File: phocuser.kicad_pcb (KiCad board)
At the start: 2 copper layers, 35 x 40 mm, 52 parts, among them J1 Conn_01x04_Male, J2 Conn_ARM_JTAG_SWD_10, J3 Conn_01x02_Male, J4 DX07S016JA1R1500, J5 Accessory 0, J6 Accessory 1, J7 Accessory 2, U1 HolyIot-18010, U2 TMC2130-LA, U3 FT231XQ

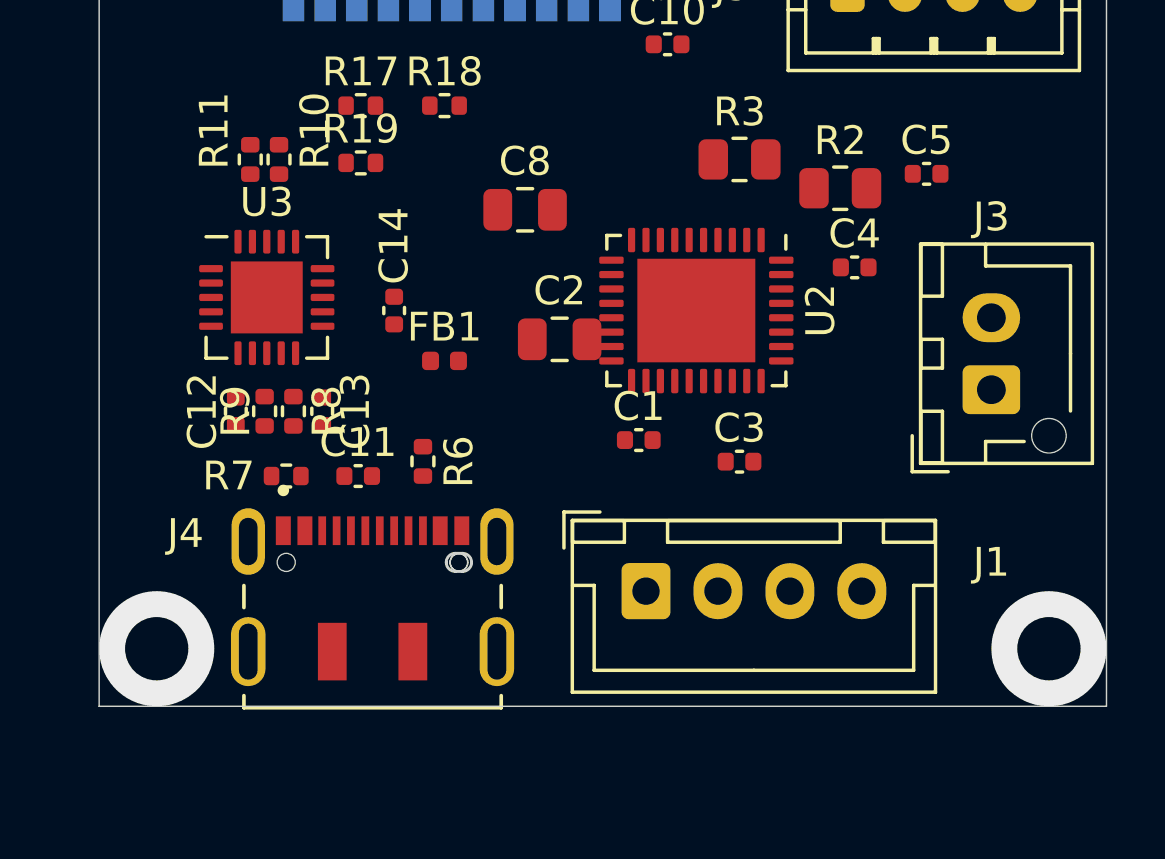
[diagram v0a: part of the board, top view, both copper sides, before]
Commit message: checkin
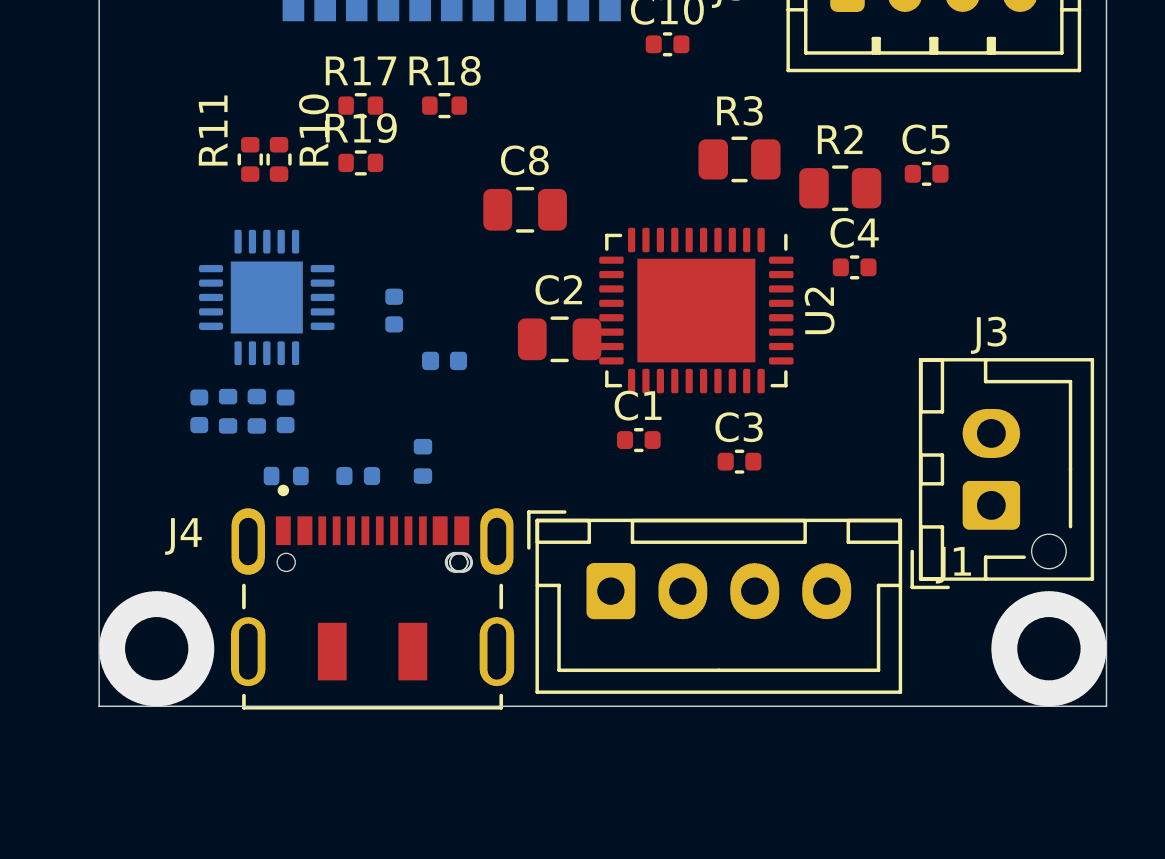
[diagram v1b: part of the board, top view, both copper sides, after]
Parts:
- C11, C12, C13, C14, FB1, R6, R7, R8, R9, U3: moved to B.Cu
- moved J3 4.02 mm to (196.0, 98.0)
- moved C12 1.27 mm to (168.5, 94.8), turned to 270 degrees
- moved C13 1.27 mm to (171.5, 94.8), turned to 90 degrees
- moved R8 1.27 mm to (170.5, 94.8), turned to 90 degrees
- moved R9 1.27 mm to (169.5, 94.8), turned to 90 degrees
- moved J1 1.22 mm to (182.8, 101.0)
- turned C14 to 90 degrees
- turned R6 to 270 degrees

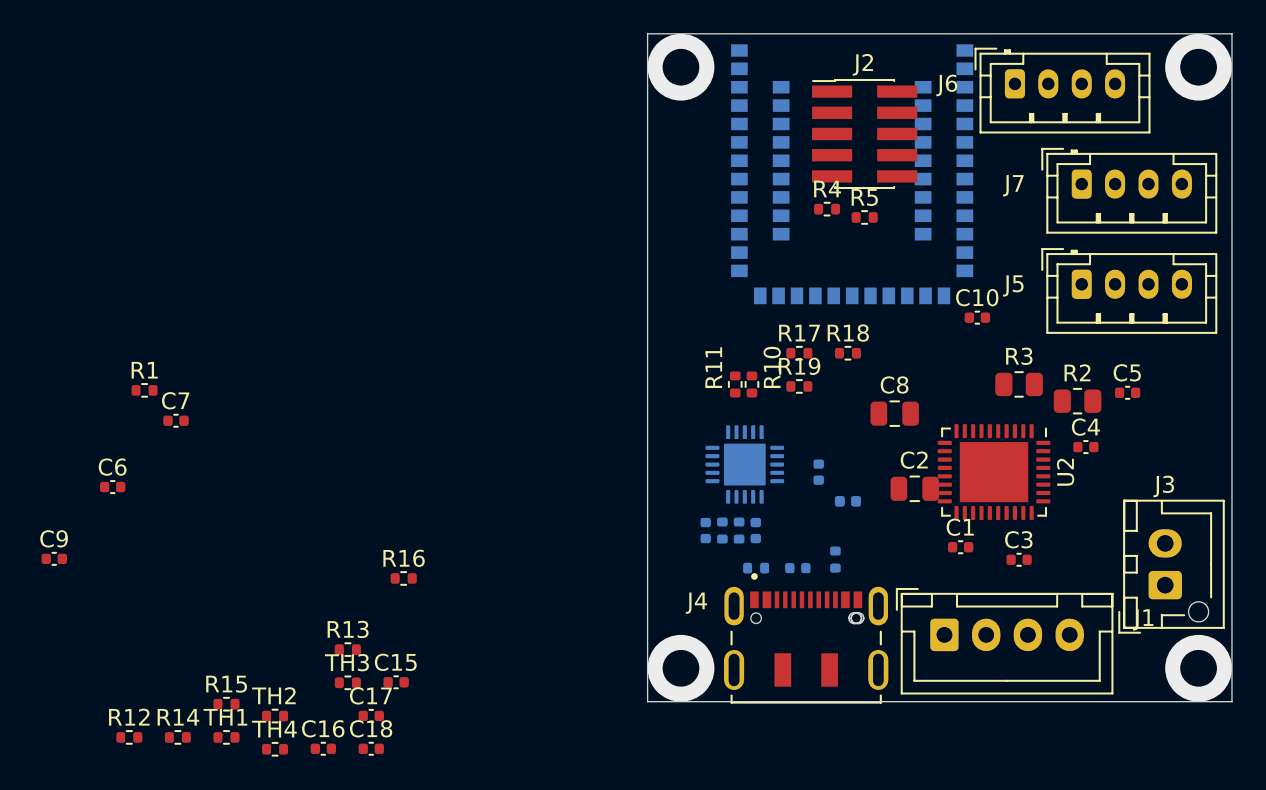
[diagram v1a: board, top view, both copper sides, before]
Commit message: Layout incremental checkin
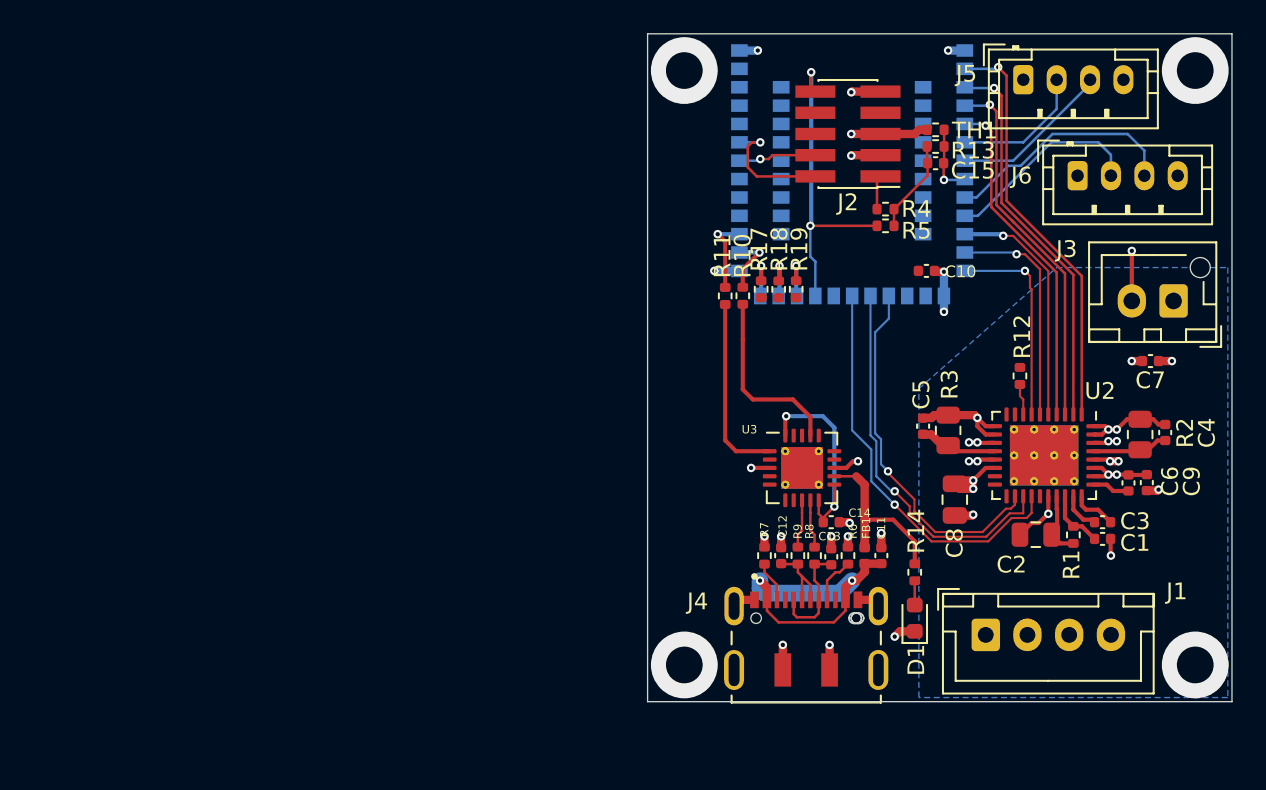
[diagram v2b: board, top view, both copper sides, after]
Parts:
- removed C16, C17, C18: 100nf, Capacitor_SMD:C_0402_1005Metric
- removed J7: Accessory 2, Connector_JST:JST_PH_B4B-PH-K_1x04_P2.00mm_Vertical
- removed R15, R16: 47k, Resistor_SMD:R_0402_1005Metric
- removed TH2, TH3, TH4: Thermistor_NTC, Resistor_SMD:R_0402_1005Metric
- added D1: LED, LED_SMD:LED_0603_1608Metric, F.Cu at (181.0, 100.0)
- C11, C12, C13, C14, FB1, R6, R7, R8, R9: moved to F.Cu
- R14: value 47k -> 470
- U2: footprint Package_DFN_QFN:QFN-36-1EP_5x6mm_P0.5mm_EP3.6x4.1mm -> Package_DFN_QFN:QFN-36-1EP_5x6mm_P0.5mm_EP3.6x4.1mm_ThermalVias
- U3: footprint Package_DFN_QFN:QFN-20-1EP_4x4mm_P0.5mm_EP2.5x2.5mm -> Package_DFN_QFN:QFN-20-1EP_4x4mm_P0.5mm_EP2.5x2.5mm_ThermalVias; moved to F.Cu
- moved C9 65.6 mm to (194.9, 91.9), turned to 270 degrees
- moved C6 60.8 mm to (193.8, 91.9), turned to 270 degrees
- moved C7 58.5 mm to (195.1, 84.6), turned to 180 degrees
- moved R12 57.6 mm to (187.3, 85.5), turned to 90 degrees
- moved R1 56.3 mm to (190.5, 95.0), turned to 90 degrees
- moved TH1 55.9 mm to (182.2, 70.8), turned to 180 degrees
- moved R13 46.3 mm to (182.2, 71.8), turned to 180 degrees
- moved R14 45.2 mm to (181.0, 97.2), turned to 90 degrees
- moved C15 44.8 mm to (182.2, 72.8)
- moved J3 17.0 mm to (196.5, 81.0), turned to 180 degrees
- moved J5 12.7 mm to (187.5, 67.8)
- moved C5 12.4 mm to (181.5, 88.5), turned to 270 degrees
- moved C1 8.51 mm to (192.2, 95.2)
- moved C2 7.75 mm to (188.2, 95.0), turned to 180 degrees
- moved J6 6.66 mm to (190.8, 73.5)
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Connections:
- C2 pad 2: GNDA -> GND
- C4 pad 2: GNDS -> GND
- C5 pad 1: GNDS -> GND
- C7 pad 2: GNDS -> GND
- C8 pad 2: GNDS -> GND
- C9 pad 2: GNDS -> GND
- J3 pad 2: GNDS -> GND
- R14 pad 1: THERM1 -> Net-(D1-Pad2)
- R14 pad 2: VCC -> VBUS
- R2 pad 1: GNDS -> GND
- R3 pad 2: GNDS -> GND
- U1 pad 10: ACC0_A -> ACC1_A
- U1 pad 11: ACC0_B -> MISO
- U1 pad 12: Net-(U1-Pad12) -> STEP
- U1 pad 13: Net-(U1-Pad13) -> DIR
- U1 pad 15: RXD -> Net-(U1-Pad15)
- U1 pad 16: TXD -> Net-(U1-Pad16)
- U1 pad 2: ACC2_A -> TMCCLK
- U1 pad 26: MISO -> TXD
- U1 pad 27: MOSI -> RXD
- U1 pad 28: SCLK -> Net-(U1-Pad28)
- U1 pad 29: ~CS1 -> Net-(U1-Pad29)
- U1 pad 3: ACC2_B -> ~CS1
- U1 pad 30: TMCCLK -> Net-(U1-Pad30)
- U1 pad 33: DIR -> Net-(U1-Pad33)
- U1 pad 34: STEP -> Net-(U1-Pad34)
- U1 pad 4: ACC1_A -> SCLK
- U1 pad 5: ACC1_B -> MOSI
- U1 pad 6: THERM0 -> ACC0_A
- U1 pad 7: THERM1 -> ACC0_B
- U1 pad 8: THERM2 -> THERM0
- U1 pad 9: THERM3 -> ACC1_B
- U2 pad 12: GNDS -> GND
- U2 pad 24: GNDA -> GND
- U2 pad 35: GNDS -> GND
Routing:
- net GND: track 0.00 -> 47.7 mm, vias 0 -> 26
- net TMCCLK: track 0.00 -> 24.9 mm, vias 0 -> 1
- net ~MOTOR_EN: track 0.00 -> 24.4 mm, vias 0 -> 1
- net ~CS1: track 0.00 -> 23.3 mm, vias 0 -> 1
- net DIAG1: track 0.00 -> 23.1 mm, vias 0 -> 1
- net SCLK: track 0.00 -> 22.1 mm, vias 0 -> 1
- net DIAG0: track 0.00 -> 21.9 mm, vias 0 -> 1
- net MOSI: track 0.00 -> 20.4 mm, vias 0 -> 1
- net ~RESET: track 0.00 -> 18.8 mm, vias 0 -> 2
- net Net-(C11-Pad1): track 0.00 -> 18.3 mm, vias 0 -> 2
- net Net-(J1-Pad1): track 0.00 -> 15.5 mm, vias 0 -> 2
- net MISO: track 0.00 -> 14.5 mm, vias 0 -> 1
- net Net-(J1-Pad4): track 0.00 -> 14.4 mm, vias 0 -> 2
- net ACC1_B: track 0.00 -> 14.2 mm
- net Net-(J1-Pad2): track 0.00 -> 14.1 mm, vias 0 -> 2
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- added copper zone on In1.Cu, net +12V
- added copper zone on B.Cu, net GND
- added copper zone on In2.Cu, net GND
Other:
- copper layers 2 -> 4
- net class Default: clearance 0.2 -> 0.1524; trace_width 0.25 -> 0.1524; via_dia 0.8 -> 0.508; via_drill 0.4 -> 0.254
- rule trace_clearance: 0.2 -> 0.1524
- rule trace_min: 0.2 -> 0.127
- rule via_min_drill: 0.3 -> 0.254
- rule via_min_size: 0.4 -> 0.508
